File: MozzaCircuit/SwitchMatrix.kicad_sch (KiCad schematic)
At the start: 94 parts, among them SW13 SW_ChocV2_rev, SW14 SW_ChocV2_rev, SW15 SW_ChocV2_rev, SW21 SW_ChocV2_rev, SW22 SW_ChocV2_rev, SW23 SW_ChocV2_rev, SW24 SW_ChocV2_rev, SW25 SW_ChocV2_rev, SW31 SW_ChocV2_rev, SW32 SW_ChocV2_rev, SW33 SW_ChocV2_rev, SW34 SW_ChocV2_rev, SW35 SW_ChocV2_rev, SW41 SW_ChocV2_rev, SW42 SW_ChocV2_rev, SW43 SW_ChocV2_rev, SW44 SW_ChocV2_rev, SW51 SW_ChocV2_rev, SW52 SW_ChocV2_rev, SW53 SW_ChocV2_rev, SW54 SW_ChocV2_rev, SW61 SW_ChocV2_rev, SW62 SW_ChocV2_rev, SW63 SW_ChocV2_rev, SW64 SW_ChocV2_rev, SW71 SW_ChocV2_rev, SW72 SW_ChocV2_rev, SW73 SW_ChocV2_rev, SW82 SW_ChocV2_rev, SW83 SW_ChocV2_rev, SW84 SW_ChocV2_rev

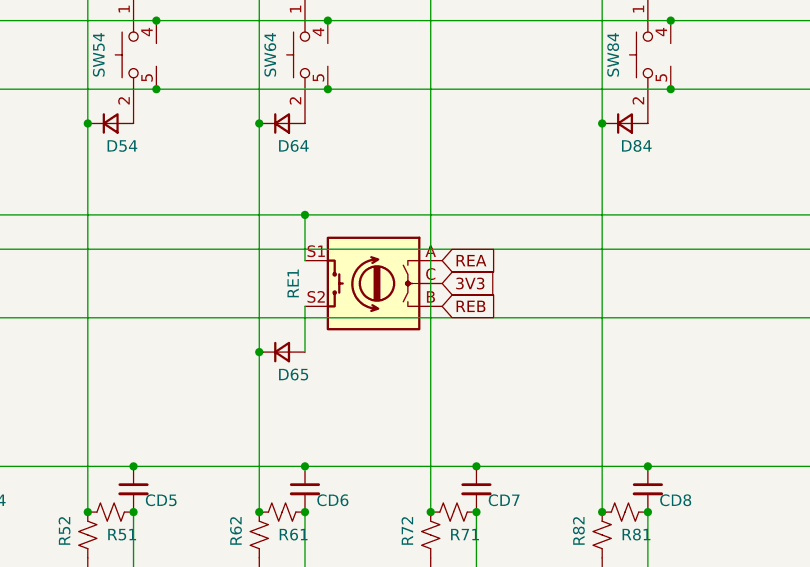
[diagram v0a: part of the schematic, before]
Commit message: rotenc diode
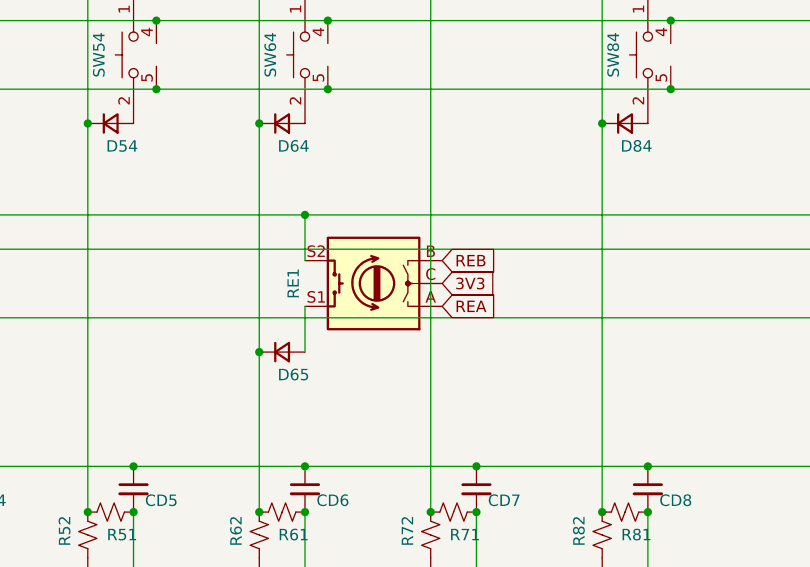
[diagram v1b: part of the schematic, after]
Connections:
- net ROW5: now also RE1.S2; no longer RE1.S1
- net at D65.2 (A): now also RE1.S1; no longer RE1.S2
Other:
- moved on the sheet: RE1
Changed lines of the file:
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@@
     )
   )
-  (global_label "REA" (shape input) (at 142.24 132.08 0) (fields_autoplaced)
-    (effects (font (size 1.27 1.27)) (justify left))
-    (property "Intersheet References" "${INTERSHEET_REFS}" (id 0) (at 148.1607 132.0006 0)
+  (global_label "REA" (shape input) (at 142.24 137.16 0) (fields_autoplaced)
+    (effects (font (size 1.27 1.27)) (justify left))
+    (property "Intersheet References" "${INTERSHEET_REFS}" (id 0) (at 148.1607 137.0806 0)
       (effects (font (size 1.27 1.27)) (justify left) hide)
     )
@@
     )
   )
-  (global_label "REB" (shape input) (at 142.24 137.16 0) (fields_autoplaced)
-    (effects (font (size 1.27 1.27)) (justify left))
-    (property "Intersheet References" "${INTERSHEET_REFS}" (id 0) (at 148.3421 137.0806 0)
+  (global_label "REB" (shape input) (at 142.24 132.08 0) (fields_autoplaced)
+    (effects (font (size 1.27 1.27)) (justify left))
+    (property "Intersheet References" "${INTERSHEET_REFS}" (id 0) (at 148.3421 132.0006 0)
       (effects (font (size 1.27 1.27)) (justify left) hide)
     )
@@
     (pin "1")
   )
-  (symbol (lib_id "Device:RotaryEncoder_Switch") (at 134.62 134.62 0) (mirror y) (unit 1)
+  (symbol (lib_id "Device:RotaryEncoder_Switch") (at 134.62 134.62 180) (unit 1)
     (in_bom yes) (on_board yes)
     (property "Reference" "RE1" (id 0) (at 125.73 134.62 90))
-    (property "Value" "RotaryEncoder_Switch" (id 1) (at 134.62 127 0)
-      (effects (font (size 1.27 1.27)) hide)
-    )
-    (property "Footprint" "00_KeyParts:RotaryEncoder_Bourns_PEC12R-4215F" (id 2) (at 138.43 130.556 0)
-      (effects (font (size 1.27 1.27)) hide)
-    )
-    (property "Datasheet" "~" (id 3) (at 134.62 128.016 0)
-      (effects (font (size 1.27 1.27)) hide)
-    )
+    (property "Value" "RotaryEncoder_Switch" (id 1) (at 134.62 142.24 0)
+      (effects (font (size 1.27 1.27)) hide)
+    )
+    (property "Footprint" "00_KeyParts:RotaryEncoder_Bourns_PEC12R-4215F" (id 2) (at 138.43 138.684 0)
+      (effects (font (size 1.27 1.27)) hide)
+    )
+    (property "Datasheet" "~" (id 3) (at 134.62 141.224 0)
+      (effects (font (size 1.27 1.27)) hide)
+    )
